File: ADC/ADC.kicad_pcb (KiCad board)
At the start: 2 copper layers, 60.4 x 70.3 mm, 145 parts, among them IC1 ADS7953SDBT, IC2 REF5025ID, IC3 ADS7953SDBT, IC4 REF5025ID, IC5 ADP3338AKCZ-5-REEL, J1 USB_C_Receptacle_USB2.0, J10 Conn_01x04_MountingPin, J11 Conn_01x04_MountingPin, J12 Conn_01x04_MountingPin, J13 Conn_01x04_MountingPin, J14 Conn_01x04_MountingPin, J15 Conn_01x02, J16 Conn_01x02, J2 Conn_01x04_MountingPin, J4 Conn_01x02, J5 Conn_01x02, J6 Conn_01x04_MountingPin, J8 Conn_01x04_MountingPin, J9 Conn_01x04_MountingPin, SW1 SW_SPDT, SW2 SW_Push, SW3 SW_Push, U1 STM32F072CBT6, U2 OPA192ID, U3 PRTR5V0U2X, U4 XC6206P332PR-G, U5 OPA192ID, U6 SHT4x, U7 LIS3MDL

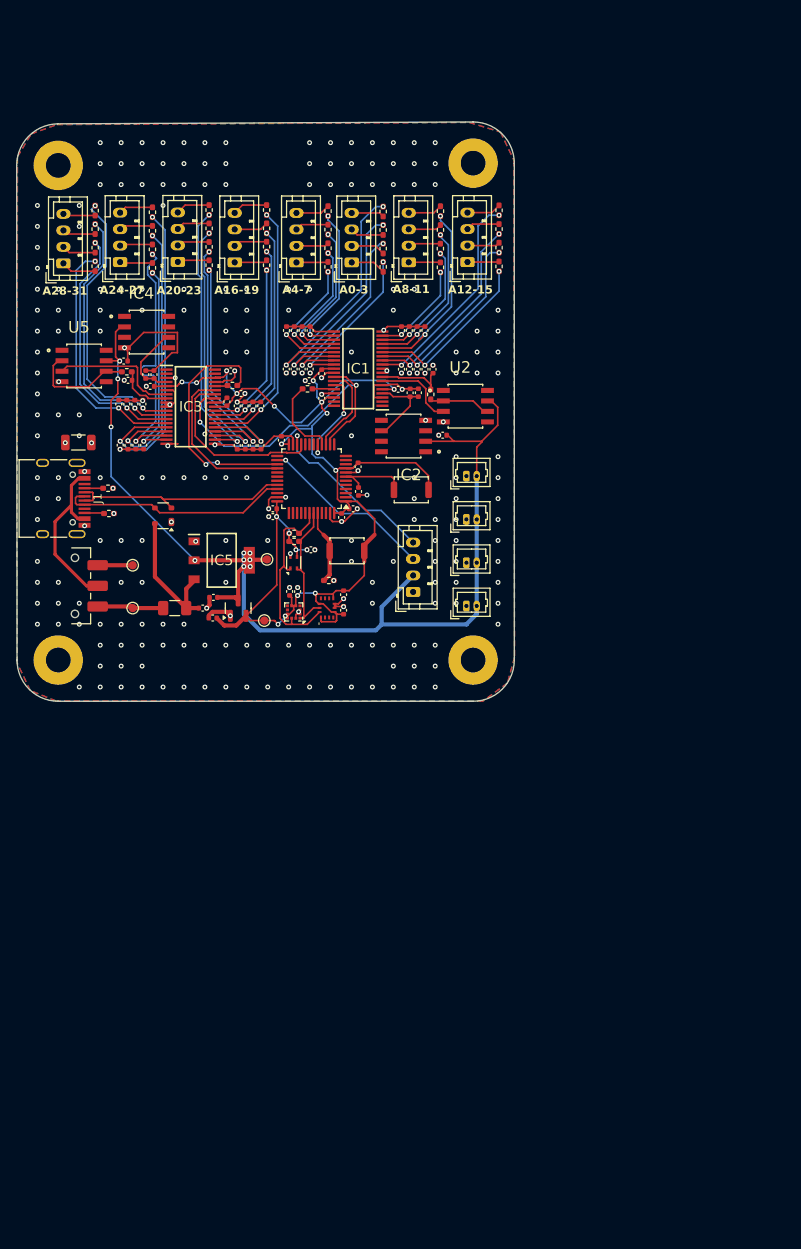
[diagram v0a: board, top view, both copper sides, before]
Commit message: finished v2
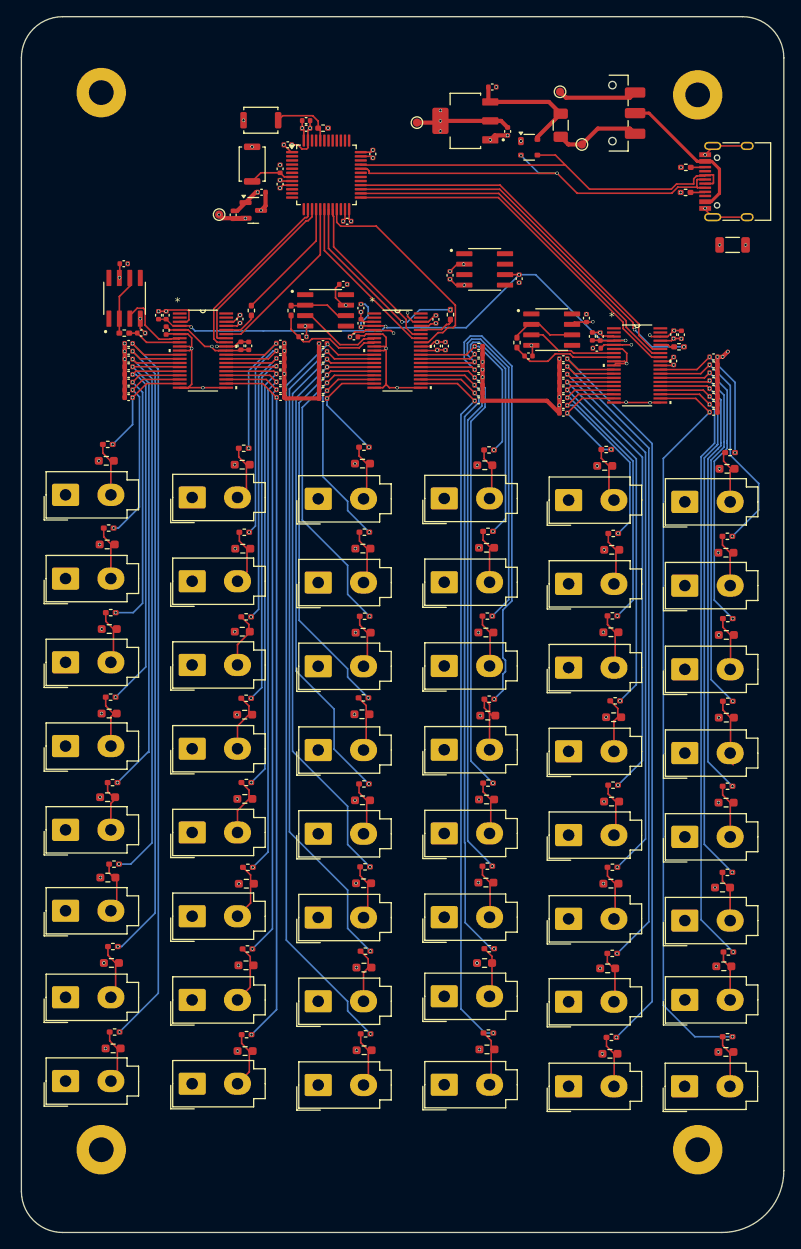
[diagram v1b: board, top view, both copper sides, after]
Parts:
- removed AC1: LSM6DSOTR, SamacSys_Parts:LGA-14_2.5X3X0.86_
- removed G***: LOGO, LOGO
- removed IC1, IC3: ADS7953SDBT, SamacSys_Parts:SOP50P640X120-38N
- removed IC2, IC4: REF5025ID, SamacSys_Parts:SOIC127P600X175-8N
- removed IC5: ADP3338AKCZ-5-REEL, SamacSys_Parts:SOT230P700X180-4N
- removed TP10, TP11, TP12, TP9: TestPoint, TestPoint:TestPoint_Pad_D1.0mm
- added C64: 270pF, Capacitor_SMD:C_0402_1005Metric, F.Cu at (59.1, 56.9)
- added C65: 270pF, Capacitor_SMD:C_0402_1005Metric, F.Cu at (59.1, 56.0)
- added C66: 270pF, Capacitor_SMD:C_0402_1005Metric, F.Cu at (59.1, 55.0)
- added C67: 270pF, Capacitor_SMD:C_0402_1005Metric, F.Cu at (59.1, 54.1)
- added C68: 270pF, Capacitor_SMD:C_0402_1005Metric, F.Cu at (59.1, 53.1)
- added C69: 270pF, Capacitor_SMD:C_0402_1005Metric, F.Cu at (59.1, 52.2)
- added C70: 270pF, Capacitor_SMD:C_0402_1005Metric, F.Cu at (106.5, 53.8)
- added C71: 270pF, Capacitor_SMD:C_0402_1005Metric, F.Cu at (106.5, 54.7)
- added C72: 270pF, Capacitor_SMD:C_0402_1005Metric, F.Cu at (106.5, 55.7)
- added C73: 270pF, Capacitor_SMD:C_0402_1005Metric, F.Cu at (106.5, 56.7)
- added C74: 270pF, Capacitor_SMD:C_0402_1005Metric, F.Cu at (106.5, 57.6)
- added C75: 270pF, Capacitor_SMD:C_0402_1005Metric, F.Cu at (106.5, 58.6)
- added C76: 270pF, Capacitor_SMD:C_0402_1005Metric, F.Cu at (106.5, 59.5)
- added C77: 270pF, Capacitor_SMD:C_0402_1005Metric, F.Cu at (106.5, 60.5)
- added C78: 270pF, Capacitor_SMD:C_0402_1005Metric, F.Cu at (88.2, 60.6)
- added C79: 270pF, Capacitor_SMD:C_0402_1005Metric, F.Cu at (88.2, 59.7)
- added C80: 270pF, Capacitor_SMD:C_0402_1005Metric, F.Cu at (88.2, 58.7)
- added C81: 270pF, Capacitor_SMD:C_0402_1005Metric, F.Cu at (88.2, 57.8)
- added C82: 270pF, Capacitor_SMD:C_0402_1005Metric, F.Cu at (88.2, 56.8)
- added C83: 270pF, Capacitor_SMD:C_0402_1005Metric, F.Cu at (88.2, 55.9)
- added C84: 270pF, Capacitor_SMD:C_0402_1005Metric, F.Cu at (88.2, 54.9)
- added C85: 270pF, Capacitor_SMD:C_0402_1005Metric, F.Cu at (88.2, 54.0)
- added J17: Conn_01x02, Connector_Molex:Molex_Mini-Fit_Jr_5566-02A_2x01_P4.20mm_Vertical, F.Cu at (27.9, 141.6)
- added J18: Conn_01x02, Connector_Molex:Molex_Mini-Fit_Jr_5566-02A_2x01_P4.20mm_Vertical, F.Cu at (73.8, 71.0)
- added J19: Conn_01x02, Connector_Molex:Molex_Mini-Fit_Jr_5566-02A_2x01_P4.20mm_Vertical, F.Cu at (73.8, 81.1)
- added J20: Conn_01x02, Connector_Molex:Molex_Mini-Fit_Jr_5566-02A_2x01_P4.20mm_Vertical, F.Cu at (73.8, 91.3)
- added J21: Conn_01x02, Connector_Molex:Molex_Mini-Fit_Jr_5566-02A_2x01_P4.20mm_Vertical, F.Cu at (73.8, 101.4)
- added J22: Conn_01x02, Connector_Molex:Molex_Mini-Fit_Jr_5566-02A_2x01_P4.20mm_Vertical, F.Cu at (73.8, 111.6)
- added J23: Conn_01x02, Connector_Molex:Molex_Mini-Fit_Jr_5566-02A_2x01_P4.20mm_Vertical, F.Cu at (73.8, 121.8)
- added J24: Conn_01x02, Connector_Molex:Molex_Mini-Fit_Jr_5566-02A_2x01_P4.20mm_Vertical, F.Cu at (73.8, 131.3)
- added J25: Conn_01x02, Connector_Molex:Molex_Mini-Fit_Jr_5566-02A_2x01_P4.20mm_Vertical, F.Cu at (73.8, 142.1)
- added J26: Conn_01x02, Connector_Molex:Molex_Mini-Fit_Jr_5566-02A_2x01_P4.20mm_Vertical, F.Cu at (58.5, 71.0)
- added J27: Conn_01x02, Connector_Molex:Molex_Mini-Fit_Jr_5566-02A_2x01_P4.20mm_Vertical, F.Cu at (58.5, 81.2)
- added J28: Conn_01x02, Connector_Molex:Molex_Mini-Fit_Jr_5566-02A_2x01_P4.20mm_Vertical, F.Cu at (58.5, 91.3)
- added J29: Conn_01x02, Connector_Molex:Molex_Mini-Fit_Jr_5566-02A_2x01_P4.20mm_Vertical, F.Cu at (58.5, 101.5)
- added J3: Conn_01x02, Connector_Molex:Molex_Mini-Fit_Jr_5566-02A_2x01_P4.20mm_Vertical, F.Cu at (43.2, 81.0)
- added J30: Conn_01x02, Connector_Molex:Molex_Mini-Fit_Jr_5566-02A_2x01_P4.20mm_Vertical, F.Cu at (58.5, 111.6)
- added J31: Conn_01x02, Connector_Molex:Molex_Mini-Fit_Jr_5566-02A_2x01_P4.20mm_Vertical, F.Cu at (58.5, 121.8)
- added J32: Conn_01x02, Connector_Molex:Molex_Mini-Fit_Jr_5566-02A_2x01_P4.20mm_Vertical, F.Cu at (58.5, 131.9)
- added J33: Conn_01x02, Connector_Molex:Molex_Mini-Fit_Jr_5566-02A_2x01_P4.20mm_Vertical, F.Cu at (58.5, 142.1)
- added J34: Conn_01x02, Connector_Molex:Molex_Mini-Fit_Jr_5566-02A_2x01_P4.20mm_Vertical, F.Cu at (103.0, 71.4)
- added J35: Conn_01x02, Connector_Molex:Molex_Mini-Fit_Jr_5566-02A_2x01_P4.20mm_Vertical, F.Cu at (103.0, 81.5)
- added J36: Conn_01x02, Connector_Molex:Molex_Mini-Fit_Jr_5566-02A_2x01_P4.20mm_Vertical, F.Cu at (103.0, 91.7)
- added J37: Conn_01x02, Connector_Molex:Molex_Mini-Fit_Jr_5566-02A_2x01_P4.20mm_Vertical, F.Cu at (103.0, 101.8)
- added J38: Conn_01x02, Connector_Molex:Molex_Mini-Fit_Jr_5566-02A_2x01_P4.20mm_Vertical, F.Cu at (103.0, 112.0)
- added J39: Conn_01x02, Connector_Molex:Molex_Mini-Fit_Jr_5566-02A_2x01_P4.20mm_Vertical, F.Cu at (103.0, 122.2)
- added J40: Conn_01x02, Connector_Molex:Molex_Mini-Fit_Jr_5566-02A_2x01_P4.20mm_Vertical, F.Cu at (103.0, 131.8)
- added J41: Conn_01x02, Connector_Molex:Molex_Mini-Fit_Jr_5566-02A_2x01_P4.20mm_Vertical, F.Cu at (103.0, 142.3)
- added J42: Conn_01x02, Connector_Molex:Molex_Mini-Fit_Jr_5566-02A_2x01_P4.20mm_Vertical, F.Cu at (88.9, 71.2)
- added J43: Conn_01x02, Connector_Molex:Molex_Mini-Fit_Jr_5566-02A_2x01_P4.20mm_Vertical, F.Cu at (88.9, 81.3)
- added J44: Conn_01x02, Connector_Molex:Molex_Mini-Fit_Jr_5566-02A_2x01_P4.20mm_Vertical, F.Cu at (88.9, 91.5)
- added J45: Conn_01x02, Connector_Molex:Molex_Mini-Fit_Jr_5566-02A_2x01_P4.20mm_Vertical, F.Cu at (88.9, 101.6)
- added J46: Conn_01x02, Connector_Molex:Molex_Mini-Fit_Jr_5566-02A_2x01_P4.20mm_Vertical, F.Cu at (88.9, 111.8)
- added J47: Conn_01x02, Connector_Molex:Molex_Mini-Fit_Jr_5566-02A_2x01_P4.20mm_Vertical, F.Cu at (88.9, 122.0)
- added J48: Conn_01x02, Connector_Molex:Molex_Mini-Fit_Jr_5566-02A_2x01_P4.20mm_Vertical, F.Cu at (88.9, 132.0)
- added J49: Conn_01x02, Connector_Molex:Molex_Mini-Fit_Jr_5566-02A_2x01_P4.20mm_Vertical, F.Cu at (88.9, 142.3)
- added J7: Conn_01x02, Connector_Molex:Molex_Mini-Fit_Jr_5566-02A_2x01_P4.20mm_Vertical, F.Cu at (43.2, 121.6)
- added R100: 33, Resistor_SMD:R_0402_1005Metric_Pad0.72x0.64mm_HandSolder, F.Cu at (94.2, 85.2)
- added R101: 33, Resistor_SMD:R_0402_1005Metric_Pad0.72x0.64mm_HandSolder, F.Cu at (94.5, 95.5)
- added R102: 33, Resistor_SMD:R_0402_1005Metric_Pad0.72x0.64mm_HandSolder, F.Cu at (94.3, 105.7)
- added R103: 33, Resistor_SMD:R_0402_1005Metric_Pad0.72x0.64mm_HandSolder, F.Cu at (94.2, 115.7)
- added R104: 33, Resistor_SMD:R_0402_1005Metric_Pad0.72x0.64mm_HandSolder, F.Cu at (94.2, 126.1)
- added R105: 33, Resistor_SMD:R_0402_1005Metric_Pad0.72x0.64mm_HandSolder, F.Cu at (94.1, 136.3)
- added R42: 33, Resistor_SMD:R_0402_1005Metric_Pad0.72x0.64mm_HandSolder, F.Cu at (33.6, 125.3)
- added R43: 33, Resistor_SMD:R_0402_1005Metric_Pad0.72x0.64mm_HandSolder, F.Cu at (33.8, 135.7)
- added R44: 33, Resistor_SMD:R_0402_1005Metric_Pad0.72x0.64mm_HandSolder, F.Cu at (79.2, 65.1)
- added R45: 33, Resistor_SMD:R_0402_1005Metric_Pad0.72x0.64mm_HandSolder, F.Cu at (79.1, 74.9)
- added R46: 1k, Resistor_SMD:R_0603_1608Metric_Pad0.98x0.95mm_HandSolder, F.Cu at (78.9, 87.2)
- added R47: 1k, Resistor_SMD:R_0603_1608Metric_Pad0.98x0.95mm_HandSolder, F.Cu at (79.1, 97.3)
- added R48: 1k, Resistor_SMD:R_0603_1608Metric_Pad0.98x0.95mm_HandSolder, F.Cu at (78.9, 107.5)
- added R49: 1k, Resistor_SMD:R_0603_1608Metric_Pad0.98x0.95mm_HandSolder, F.Cu at (78.9, 117.5)
- added R50: 1k, Resistor_SMD:R_0603_1608Metric_Pad0.98x0.95mm_HandSolder, F.Cu at (78.7, 127.3)
- added R51: 1k, Resistor_SMD:R_0603_1608Metric_Pad0.98x0.95mm_HandSolder, F.Cu at (79.0, 137.8)
- added R52: 33, Resistor_SMD:R_0402_1005Metric_Pad0.72x0.64mm_HandSolder, F.Cu at (79.0, 85.2)
- added R53: 33, Resistor_SMD:R_0402_1005Metric_Pad0.72x0.64mm_HandSolder, F.Cu at (79.3, 95.3)
- added R54: 33, Resistor_SMD:R_0402_1005Metric_Pad0.72x0.64mm_HandSolder, F.Cu at (79.1, 105.5)
- added R55: 33, Resistor_SMD:R_0402_1005Metric_Pad0.72x0.64mm_HandSolder, F.Cu at (79.0, 115.6)
- added R56: 33, Resistor_SMD:R_0402_1005Metric_Pad0.72x0.64mm_HandSolder, F.Cu at (79.3, 125.6)
- added R57: 33, Resistor_SMD:R_0402_1005Metric_Pad0.72x0.64mm_HandSolder, F.Cu at (79.2, 135.8)
- added R58: 1k, Resistor_SMD:R_0603_1608Metric_Pad0.98x0.95mm_HandSolder, F.Cu at (63.9, 66.7)
- added R59: 1k, Resistor_SMD:R_0603_1608Metric_Pad0.98x0.95mm_HandSolder, F.Cu at (63.9, 77.0)
- added R60: 1k, Resistor_SMD:R_0603_1608Metric_Pad0.98x0.95mm_HandSolder, F.Cu at (64.0, 87.2)
- added R61: 1k, Resistor_SMD:R_0603_1608Metric_Pad0.98x0.95mm_HandSolder, F.Cu at (63.8, 97.1)
- added R62: 1k, Resistor_SMD:R_0603_1608Metric_Pad0.98x0.95mm_HandSolder, F.Cu at (63.9, 107.6)
- added R63: 1k, Resistor_SMD:R_0603_1608Metric_Pad0.98x0.95mm_HandSolder, F.Cu at (64.0, 117.6)
- added R64: 33, Resistor_SMD:R_0402_1005Metric_Pad0.72x0.64mm_HandSolder, F.Cu at (64.1, 64.7)
- added R65: 33, Resistor_SMD:R_0402_1005Metric_Pad0.72x0.64mm_HandSolder, F.Cu at (64.1, 75.0)
- added R66: 33, Resistor_SMD:R_0402_1005Metric_Pad0.72x0.64mm_HandSolder, F.Cu at (64.1, 85.2)
- added R67: 33, Resistor_SMD:R_0402_1005Metric_Pad0.72x0.64mm_HandSolder, F.Cu at (64.0, 95.1)
- added R68: 33, Resistor_SMD:R_0402_1005Metric_Pad0.72x0.64mm_HandSolder, F.Cu at (64.1, 105.6)
- added R69: 33, Resistor_SMD:R_0402_1005Metric_Pad0.72x0.64mm_HandSolder, F.Cu at (64.2, 115.6)
- added R70: 1k, Resistor_SMD:R_0603_1608Metric_Pad0.98x0.95mm_HandSolder, F.Cu at (64.1, 127.9)
- added R71: 1k, Resistor_SMD:R_0603_1608Metric_Pad0.98x0.95mm_HandSolder, F.Cu at (64.1, 137.9)
- added R72: 1k, Resistor_SMD:R_0603_1608Metric_Pad0.98x0.95mm_HandSolder, F.Cu at (108.1, 67.3)
- added R73: 1k, Resistor_SMD:R_0603_1608Metric_Pad0.98x0.95mm_HandSolder, F.Cu at (108.0, 77.5)
- added R74: 1k, Resistor_SMD:R_0603_1608Metric_Pad0.98x0.95mm_HandSolder, F.Cu at (108.0, 87.5)
- added R75: 1k, Resistor_SMD:R_0603_1608Metric_Pad0.98x0.95mm_HandSolder, F.Cu at (108.0, 97.5)
- added R76: 33, Resistor_SMD:R_0402_1005Metric_Pad0.72x0.64mm_HandSolder, F.Cu at (64.2, 125.9)
- added R77: 33, Resistor_SMD:R_0402_1005Metric_Pad0.72x0.64mm_HandSolder, F.Cu at (64.3, 135.9)
- added R78: 33, Resistor_SMD:R_0402_1005Metric_Pad0.72x0.64mm_HandSolder, F.Cu at (108.5, 65.4)
- added R79: 33, Resistor_SMD:R_0402_1005Metric_Pad0.72x0.64mm_HandSolder, F.Cu at (108.2, 75.5)
- added R80: 33, Resistor_SMD:R_0402_1005Metric_Pad0.72x0.64mm_HandSolder, F.Cu at (108.2, 85.5)
- added R81: 33, Resistor_SMD:R_0402_1005Metric_Pad0.72x0.64mm_HandSolder, F.Cu at (108.2, 95.5)
- added R82: 1k, Resistor_SMD:R_0603_1608Metric_Pad0.98x0.95mm_HandSolder, F.Cu at (108.0, 107.8)
- added R83: 1k, Resistor_SMD:R_0603_1608Metric_Pad0.98x0.95mm_HandSolder, F.Cu at (107.6, 118.2)
- added R84: 1k, Resistor_SMD:R_0603_1608Metric_Pad0.98x0.95mm_HandSolder, F.Cu at (107.7, 127.7)
- added R85: 1k, Resistor_SMD:R_0603_1608Metric_Pad0.98x0.95mm_HandSolder, F.Cu at (108.0, 138.1)
- added R86: 1k, Resistor_SMD:R_0603_1608Metric_Pad0.98x0.95mm_HandSolder, F.Cu at (93.3, 67.0)
- added R87: 1k, Resistor_SMD:R_0603_1608Metric_Pad0.98x0.95mm_HandSolder, F.Cu at (94.1, 77.2)
- added R88: 33, Resistor_SMD:R_0402_1005Metric_Pad0.72x0.64mm_HandSolder, F.Cu at (108.2, 105.9)
- added R89: 33, Resistor_SMD:R_0402_1005Metric_Pad0.72x0.64mm_HandSolder, F.Cu at (108.2, 116.3)
- added R90: 33, Resistor_SMD:R_0402_1005Metric_Pad0.72x0.64mm_HandSolder, F.Cu at (108.3, 126.0)
- added R91: 33, Resistor_SMD:R_0402_1005Metric_Pad0.72x0.64mm_HandSolder, F.Cu at (108.2, 136.2)
- added R92: 33, Resistor_SMD:R_0402_1005Metric_Pad0.72x0.64mm_HandSolder, F.Cu at (93.5, 65.0)
- added R93: 33, Resistor_SMD:R_0402_1005Metric_Pad0.72x0.64mm_HandSolder, F.Cu at (94.3, 75.2)
- added R94: 1k, Resistor_SMD:R_0603_1608Metric_Pad0.98x0.95mm_HandSolder, F.Cu at (94.0, 87.2)
- added R95: 1k, Resistor_SMD:R_0603_1608Metric_Pad0.98x0.95mm_HandSolder, F.Cu at (94.4, 97.5)
- added R96: 1k, Resistor_SMD:R_0603_1608Metric_Pad0.98x0.95mm_HandSolder, F.Cu at (94.1, 107.7)
- added R97: 1k, Resistor_SMD:R_0603_1608Metric_Pad0.98x0.95mm_HandSolder, F.Cu at (94.0, 117.7)
- added R98: 1k, Resistor_SMD:R_0603_1608Metric_Pad0.98x0.95mm_HandSolder, F.Cu at (93.6, 128.0)
- added R99: 1k, Resistor_SMD:R_0603_1608Metric_Pad0.98x0.95mm_HandSolder, F.Cu at (93.9, 138.3)
- added TP1: TestPoint, TestPoint:TestPoint_Pad_D1.0mm, F.Cu at (87.8, 21.6)
- added TP2: TestPoint, TestPoint:TestPoint_Pad_D1.0mm, F.Cu at (90.5, 28.0)
- added TP3: TestPoint, TestPoint:TestPoint_Pad_D1.0mm, F.Cu at (46.5, 36.5)
- added TP4: TestPoint, TestPoint:TestPoint_Pad_D1.0mm, F.Cu at (70.5, 25.4)
- added U10: XC6206P332PR-G, Package_TO_SOT_SMD:SOT-23, F.Cu at (50.6, 36.0)
- added U11: ADP3338AKCZ-5-REEL, footprint:SOT230P700X180-4N, F.Cu at (76.4, 25.1)
- added U8: OPA192ID, footprint:SOIC127P599X175-8N, F.Cu at (35.0, 46.7)
- added U9: REF5025ID, footprint:SOIC127P599X175-8N, F.Cu at (78.7, 43.2)
- C11, C12: value 1uF -> 100nF
- C13, C14, C15, C19, C23, C24, C25: value 270pF -> 100nF
- C16, C20, C21, C22: value 270pF -> 10uF
- C17, C18, C26, C27, C28, C29, C30, C31, C36, C37: value 270pF -> 1uF
- C2, C3: value 100nF -> 1uF
- C42, C59, C60: value 1uF -> 270pF
- C49, C50, C51, C63: value 10uF -> 270pF
- C52, C53, C54, C55, C57, C58, C61, C62: value 100nF -> 270pF
- C56: value 220nF -> 270pF
- C7, C8: value 100nF -> 10uF
- J10, J11, J12, J13, J14, J2, J6, J8, J9: value Conn_01x04_MountingPin -> Conn_01x02; footprint Connector_JST:JST_PH_B4B-PH-K_1x04_P2.00mm_Vertical -> Connector_Molex:Molex_Mini-Fit_Jr_5566-02A_2x01_P4.20mm_Vertical
- J15, J16, J4, J5: footprint Connector_Molex:Molex_PicoBlade_53047-0210_1x02_P1.25mm_Vertical -> Connector_Molex:Molex_Mini-Fit_Jr_5566-02A_2x01_P4.20mm_Vertical
- R10, R11, R12, R13, R14, R15, R22, R23, R24, R25, R26, R27, R34, R35, R36, R37, R38, R39: value 33 -> 1k; footprint Resistor_SMD:R_0402_1005Metric_Pad0.72x0.64mm_HandSolder -> Resistor_SMD:R_0603_1608Metric_Pad0.98x0.95mm_HandSolder
- R2, R3: value 5.1k -> 33
- R5: value 33 -> 5.1k
- R6: value 10k -> 5.1k
- R7: value 10k -> 33
- SW1: value SW_SPDT -> SW_Push; footprint Button_Switch_SMD:SW_SPDT_CK_JS102011SAQN -> Button_Switch_SMD:SW_Push_SPST_NO_Alps_SKRK
- SW3: value SW_Push -> SW_SPDT; footprint Button_Switch_SMD:SW_Push_SPST_NO_Alps_SKRK -> Button_Switch_SMD:SW_SPDT_CK_JS102011SAQN
- U2: value OPA192ID -> ADS7953SDBT; footprint SamacSys_Parts:SOIC127P600X175-8N -> footprint:DBT38
- U3: value PRTR5V0U2X -> ADS7953SDBT; footprint Package_TO_SOT_SMD:SOT-143 -> footprint:DBT38
- U4: value XC6206P332PR-G -> ADS7953SDBT; footprint Package_TO_SOT_SMD:SOT-23 -> footprint:DBT38
- U5: footprint SamacSys_Parts:SOIC127P600X175-8N -> footprint:SOIC127P599X175-8N
- U6: value SHT4x -> PRTR5V0U2X; footprint Sensor_Humidity:Sensirion_DFN-4_1.5x1.5mm_P0.8mm_SHT4x_NoCentralPad -> Package_TO_SOT_SMD:SOT-143
- U7: value LIS3MDL -> OPA192ID; footprint Package_LGA:LGA-12_2x2mm_P0.5mm -> footprint:SOIC127P599X175-8N
- moved H3 122.8 mm to (104.5, 150.0)
- moved R23 106.5 mm to (49.6, 138.0), turned to 0 degrees
- moved J9 103.1 mm to (43.2, 141.9)
- moved R37 97.2 mm to (33.6, 137.7), turned to 0 degrees
- moved R29 95.7 mm to (49.8, 136.0), turned to 0 degrees
- moved R22 94.5 mm to (49.8, 127.6), turned to 0 degrees
- moved J1 91.8 mm to (109.5, 32.5), turned to 90 degrees
- moved J8 90.4 mm to (43.2, 131.8)
- moved R36 84.5 mm to (33.4, 127.3), turned to 0 degrees
- moved R28 83.1 mm to (49.9, 125.6), turned to 0 degrees
- moved L1 82.9 mm to (108.8, 40.2), turned to 0 degrees
- moved H4 82.3 mm to (32.2, 21.7)
- moved R15 82.2 mm to (49.8, 117.7), turned to 0 degrees
- moved R21 81.1 mm to (50.0, 115.7), turned to 0 degrees
- moved R35 80.9 mm to (33.0, 116.9), turned to 0 degrees
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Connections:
- C1 pad 1: +3.3V -> +5V
- C10 pad 1: /VBUS_fuse -> +3.3V
- C11 pad 1: GND -> +3.3V
- C11 pad 2: +5V -> GND
- C12 pad 1: GND -> +3.3V
- C12 pad 2: +3.3V -> GND
- C13 pad 1: OUT_AMP1 -> NRST
- C14 pad 1: A15 -> +3.3V
- C15 pad 1: A14 -> +3.3V
- C16 pad 1: A13 -> +3.3V
- C17 pad 1: A12 -> +5V
- C18 pad 1: A11 -> +5V
- C19 pad 1: A10 -> +5V
- C2 pad 1: +3.3V -> +5V
- C20 pad 1: A9 -> GND
- C20 pad 2: GND -> +5V
- C21 pad 1: A7 -> GND
- C21 pad 2: GND -> +5V
- C22 pad 1: A6 -> GND
- C22 pad 2: GND -> +5V
- C23 pad 1: A5 -> GND
- C23 pad 2: GND -> +5V
- C24 pad 1: A4 -> GND
- C24 pad 2: GND -> +5V
- C25 pad 1: A3 -> GND
- C25 pad 2: GND -> +5V
- C26 pad 1: A2 -> +5V
- C27 pad 1: A1 -> /VBUS_fuse
- C28 pad 1: A0 -> +5V
- C29 pad 1: A31 -> +5V
- C3 pad 1: +3.3V -> +5V
- C30 pad 1: A30 -> REFIN
- C31 pad 1: A29 -> +5V
- C32 pad 1: A28 -> OUT_AMP3
- C33 pad 1: +3.3V -> GND
- C33 pad 2: GND -> +5V
- C34 pad 1: A27 -> OUT_AMP2
- C35 pad 1: A26 -> OUT_AMP1
- C36 pad 1: A25 -> GND
- C36 pad 2: GND -> +3.3V
- C37 pad 1: A23 -> +5V
- C38 pad 1: A22 -> A0
- C39 pad 1: A21 -> A1
- C4 pad 1: +3.3V -> GND
- C4 pad 2: GND -> REFIN
- C40 pad 1: A20 -> A2
- C41 pad 1: A19 -> A3
- C42 pad 1: +3.3V -> A4
- C43 pad 1: A18 -> A5
- C44 pad 1: A17 -> A6
- C45 pad 1: A16 -> A7
- C46 pad 1: OUT_AMP2 -> A8
- C47 pad 1: A24 -> A9
- C48 pad 1: A8 -> A10
- C49 pad 1: GND -> A11
- C49 pad 2: REFIN1 -> GND
- C5 pad 1: NRST -> GND
- C5 pad 2: GND -> REFIN
- C50 pad 1: GND -> A12
- C50 pad 2: +3.3V -> GND
- C51 pad 1: GND -> A13
- C51 pad 2: +3.3V -> GND
- C52 pad 1: GND -> A14
- C52 pad 2: REFIN2 -> GND
- C53 pad 1: GND -> A15
- C53 pad 2: +3.3V -> GND
- C54 pad 1: GND -> A16
- C54 pad 2: +3.3V -> GND
- C55 pad 1: GND -> A17
- C55 pad 2: REFIN1 -> GND
- C56 pad 1: GND -> A18
- C56 pad 2: +3.3V -> GND
- C57 pad 1: GND -> A19
- C57 pad 2: +3.3V -> GND
- C58 pad 1: GND -> A20
- C58 pad 2: +3.3V -> GND
- C59 pad 1: +5V -> A21
- C6 pad 1: +3.3V -> GND
- C6 pad 2: GND -> REFIN
- C60 pad 1: +5V -> A22
- C61 pad 1: GND -> A23
- C61 pad 2: +3.3V -> GND
- C62 pad 1: GND -> A24
- C62 pad 2: +3.3V -> GND
- C63 pad 1: GND -> A25
- C63 pad 2: REFIN2 -> GND
- C7 pad 1: +3.3V -> GND
- C7 pad 2: GND -> REFIN
- C8 pad 1: +3.3V -> GND
- C8 pad 2: GND -> REFIN
- C9 pad 1: +3.3V -> GND
- C9 pad 2: GND -> REFIN
- J10 pad 1: Net-(J10-Pin_1) -> GND
- J11 pad 1: Net-(J11-Pin_1) -> GND
- J12 pad 1: Net-(J12-Pin_1) -> GND
- J13 pad 1: Net-(J13-Pin_1) -> GND
- J14 pad 1: Net-(J14-Pin_1) -> GND
- J15 pad 2: +5V -> Net-(J15-Pin_2)
- J16 pad 2: +5V -> Net-(J16-Pin_2)
- J2 pad 1: Net-(J2-Pin_1) -> GND
- J4 pad 2: +5V -> Net-(J4-Pin_2)
- J5 pad 2: +5V -> Net-(J5-Pin_2)
- J6 pad 2: +5V -> Net-(J6-Pin_2)
- J8 pad 1: Net-(J8-Pin_1) -> GND
- J9 pad 1: Net-(J9-Pin_1) -> GND
- R10 pad 1: A2 -> +5V
- R10 pad 2: Net-(J2-Pin_3) -> Net-(J2-Pin_2)
- R11 pad 1: A3 -> +5V
- R11 pad 2: Net-(J2-Pin_4) -> Net-(J3-Pin_2)
- R12 pad 1: A4 -> +5V
- R12 pad 2: Net-(J8-Pin_1) -> Net-(J4-Pin_2)
- R13 pad 1: A5 -> +5V
- R13 pad 2: Net-(J8-Pin_2) -> Net-(J5-Pin_2)
- R14 pad 1: A6 -> +5V
- R14 pad 2: Net-(J8-Pin_3) -> Net-(J6-Pin_2)
- R15 pad 1: A7 -> +5V
- R15 pad 2: Net-(J8-Pin_4) -> Net-(J7-Pin_2)
- R16 pad 1: A8 -> Net-(J2-Pin_2)
- R16 pad 2: Net-(J9-Pin_1) -> A0
- R17 pad 1: A9 -> Net-(J3-Pin_2)
- R17 pad 2: Net-(J9-Pin_2) -> A1
- R18 pad 1: A10 -> Net-(J4-Pin_2)
- R18 pad 2: Net-(J9-Pin_3) -> A2
- R19 pad 1: A11 -> Net-(J5-Pin_2)
- R19 pad 2: Net-(J9-Pin_4) -> A3
- R2 pad 1: GND -> Net-(U2-SDO)
- R2 pad 2: Net-(J1-CC1) -> MISO_SPI1
- R20 pad 1: A12 -> Net-(J6-Pin_2)
- R20 pad 2: Net-(J10-Pin_1) -> A4
- R21 pad 1: A13 -> Net-(J7-Pin_2)
- R21 pad 2: Net-(J10-Pin_2) -> A5
- R22 pad 1: A14 -> +5V
- R22 pad 2: Net-(J10-Pin_3) -> Net-(J8-Pin_2)
- R23 pad 1: A15 -> +5V
- R23 pad 2: Net-(J10-Pin_4) -> Net-(J9-Pin_2)
- R24 pad 1: Net-(J12-Pin_1) -> +5V
- R24 pad 2: A16 -> Net-(J10-Pin_2)
- R25 pad 1: Net-(J12-Pin_2) -> +5V
- R25 pad 2: A17 -> Net-(J11-Pin_2)
- R26 pad 1: Net-(J12-Pin_3) -> +5V
- R26 pad 2: A18 -> Net-(J12-Pin_2)
- R27 pad 1: Net-(J12-Pin_4) -> +5V
- R27 pad 2: A19 -> Net-(J13-Pin_2)
- R28 pad 1: Net-(J11-Pin_1) -> Net-(J8-Pin_2)
- R28 pad 2: A20 -> A6
- R29 pad 1: Net-(J11-Pin_2) -> Net-(J9-Pin_2)
- R29 pad 2: A21 -> A7
- R3 pad 1: GND -> Net-(U3-SDO)
- R3 pad 2: Net-(J1-CC2) -> MISO_SPI2
- R30 pad 1: Net-(J11-Pin_3) -> Net-(J10-Pin_2)
- R30 pad 2: A22 -> A8
- R31 pad 1: Net-(J11-Pin_4) -> Net-(J11-Pin_2)
- R31 pad 2: A23 -> A9
- R32 pad 1: Net-(J13-Pin_1) -> Net-(J12-Pin_2)
- R32 pad 2: A24 -> A10
- R33 pad 2: A25 -> A11
- R34 pad 1: Net-(J13-Pin_3) -> +5V
- R34 pad 2: A26 -> Net-(J14-Pin_2)
- R35 pad 1: Net-(J13-Pin_4) -> +5V
- R35 pad 2: A27 -> Net-(J15-Pin_2)
- R36 pad 1: Net-(J14-Pin_1) -> +5V
- R36 pad 2: A28 -> Net-(J16-Pin_2)
- R37 pad 1: Net-(J14-Pin_2) -> +5V
- R37 pad 2: A29 -> Net-(J17-Pin_2)
- R38 pad 1: Net-(J14-Pin_3) -> +5V
- R38 pad 2: A30 -> Net-(J18-Pin_2)
- R39 pad 1: Net-(J14-Pin_4) -> +5V
- R39 pad 2: A31 -> Net-(J19-Pin_2)
- R4 pad 1: Net-(U2--IN) -> Net-(U4-SDO)
- R4 pad 2: OUT_AMP1 -> MISO_SPI3
- R40 pad 1: Net-(IC1-SDO) -> Net-(J14-Pin_2)
- R40 pad 2: MISO_SPI1 -> A12
- R41 pad 1: Net-(IC3-SDO) -> Net-(J15-Pin_2)
- R41 pad 2: MISO_SPI2 -> A13
- R5 pad 1: Net-(U5--IN) -> GND
- R5 pad 2: OUT_AMP2 -> Net-(J1-CC1)
- R6 pad 1: +3.3V -> GND
- R6 pad 2: SDA_I2C1 -> Net-(J1-CC2)
- R7 pad 1: +3.3V -> Net-(U5--IN)
- R7 pad 2: SCL_I2C1 -> OUT_AMP3
- R8 pad 1: A0 -> Net-(U7--IN)
- R8 pad 2: Net-(J2-Pin_1) -> OUT_AMP2
- R9 pad 1: A1 -> Net-(U8--IN)
- R9 pad 2: Net-(J2-Pin_2) -> OUT_AMP1
- SW1 pad 1: Net-(SW1-A) -> +3.3V
- SW1 pad 2: VBUS -> BOOT0
- SW3 pad 1: +3.3V -> Net-(SW3-A)
- SW3 pad 2: BOOT0 -> VBUS
- U1 pad 14: CS_SPI -> CS_SPI1
- U1 pad 18: unconnected-(U1-PB0-Pad18) -> SCK_SPI3
- U1 pad 19: unconnected-(U1-PB1-Pad19) -> MISO_SPI3
- U1 pad 20: unconnected-(U1-PB2-Pad20) -> MOSI_SPI3
- U1 pad 21: SCK_SPI2 -> CS_SPI3
- U1 pad 22: SDA_I2C2 -> unconnected-(U1-PB11-Pad22)
- U1 pad 25: unconnected-(U1-PB12-Pad25) -> CS_SPI2
- U1 pad 26: SCL_I2C2 -> SCK_SPI2
- U1 pad 42: SDA_I2C1 -> unconnected-(U1-PB6-Pad42)
- U1 pad 43: SCL_I2C1 -> unconnected-(U1-PB7-Pad43)
- U2 pad 2: Net-(U2--IN) -> unconnected-(U2-GPIO3-Pad2)
- U2 pad 3: +AMP1 -> GND
- U2 pad 4: GND -> REFIN
- U2 pad 5: unconnected-(U2-NC_2-Pad5) -> +5V
- U2 pad 6: Net-(U2--IN) -> GND
- U2 pad 7: +5V -> +AMP1
- U2 pad 8: unconnected-(U2-NC_3-Pad8) -> OUT_AMP1
- U3 pad 1: GND -> unconnected-(U3-GPIO2-Pad1)
- U3 pad 2: D_N -> unconnected-(U3-GPIO3-Pad2)
- U3 pad 3: D_P -> GND
- U3 pad 4: /VBUS_fuse -> REFIN
- U4 pad 1: GND -> unconnected-(U4-GPIO2-Pad1)
- U4 pad 2: +3.3V -> unconnected-(U4-GPIO3-Pad2)
- U4 pad 3: +5V -> GND
- U5 pad 1: unconnected-(U5-NC_1-Pad1) -> (no net)
- U5 pad 3: +AMP2 -> +AMP3
- U5 pad 5: unconnected-(U5-NC_2-Pad5) -> (no net)
- U5 pad 8: unconnected-(U5-NC_3-Pad8) -> (no net)
- U6 pad 1: SDA_I2C1 -> GND
- U6 pad 2: SCL_I2C1 -> D_N
- U6 pad 3: +3.3V -> D_P
- U6 pad 4: GND -> /VBUS_fuse
- U7 pad 1: SCL_I2C1 -> (no net)
- U7 pad 2: GND -> Net-(U7--IN)
- U7 pad 3: GND -> +AMP2
- U7 pad 4: unconnected-(U7-C1-Pad4) -> GND
- U7 pad 5: +3.3V -> (no net)
- U7 pad 6: +3.3V -> Net-(U7--IN)
- U7 pad 7: unconnected-(U7-INT-Pad7) -> +5V
- U7 pad 8: unconnected-(U7-DRDY-Pad8) -> (no net)
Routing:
- net +3.3V: track 159.9 -> 13.6 mm, vias 19 -> 9
- net A47: track 0.00 -> 94.6 mm, vias 0 -> 2
- net A39: track 0.00 -> 90.9 mm, vias 0 -> 2
- net A46: track 0.00 -> 82.9 mm, vias 0 -> 2
- net REFIN: track 0.00 -> 76.2 mm, vias 0 -> 6
- net A38: track 0.00 -> 75.5 mm, vias 0 -> 2
- net A45: track 0.00 -> 71.0 mm, vias 0 -> 2
- net GND: track 97.6 -> 166.4 mm, vias 258 -> 65
- net A15: track 26.2 -> 93.1 mm
- net A37: track 0.00 -> 66.5 mm, vias 0 -> 2
- net A7: track 19.4 -> 85.4 mm
- net A31: track 34.2 -> 96.3 mm
- net A44: track 0.00 -> 59.6 mm, vias 0 -> 2
- net A14: track 24.1 -> 81.6 mm
- net A6: track 18.4 -> 75.7 mm
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- added copper zone on In1.Cu, net +3.3V
- added copper zone on In1.Cu, net +5V
- added copper zone on In2.Cu, net GND
- removed copper zone on B.Cu, net GND
- removed copper zone on F.Cu, net GND
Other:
- board size 60.4 x 70.3 mm -> 92.5 x 147.5 mm
- copper layers 2 -> 4
- board text removed: "A0-3"
- board text removed: "A12-15"
- board text removed: "A16-19"
- board text removed: "A20-23"
- board text removed: "A24-27"
- board text removed: "A28-31"
- board text removed: "A4-7"
- board text removed: "A8-11"
- board text removed: "Aramaki Lab"
- board text removed: "Designed by Madhav Kapa"
